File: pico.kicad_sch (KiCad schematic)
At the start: 43 parts, among them J101 Programming, J102 ???, J103 XT60, J104 Conn_01x03, Q101 AGM30P100D, Q102 BSS138, Q103 AGM30P100D, Q104 AGM30P100D, Q105 AGM30P100D, Q106 AGM30P100D, U101 TPS7A2033PDBVR, U106 ADC124S051CIMM/NOPB

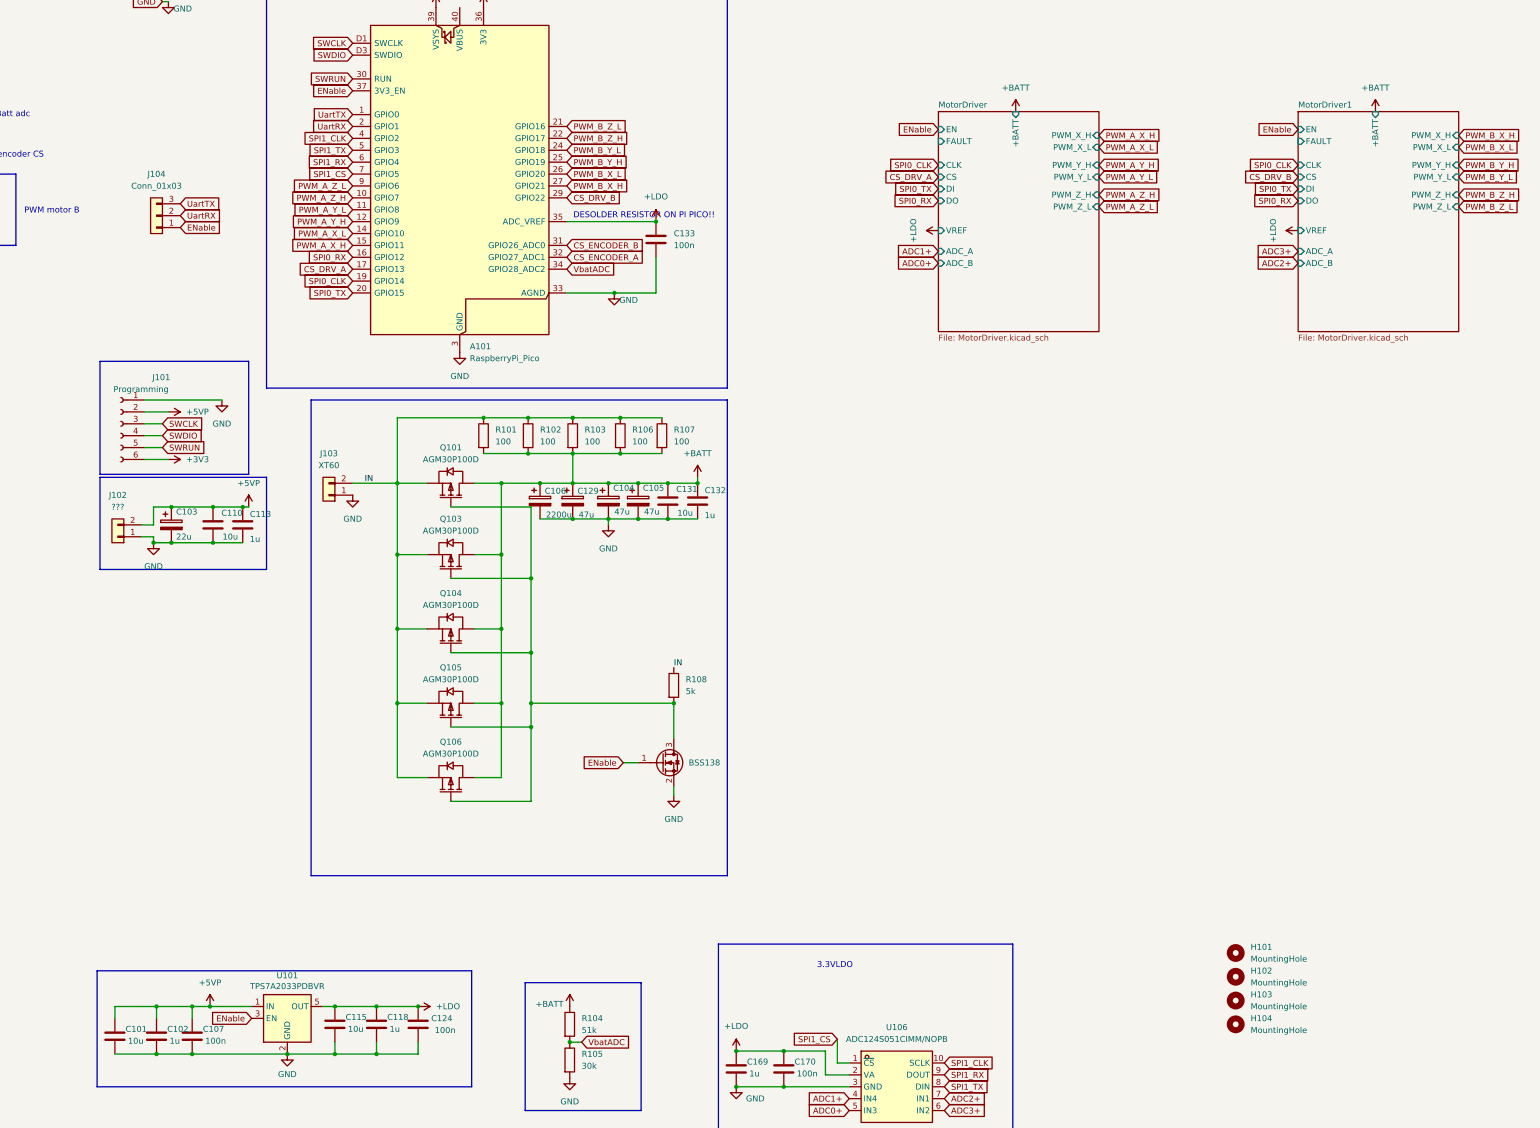
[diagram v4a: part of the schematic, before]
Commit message: done?
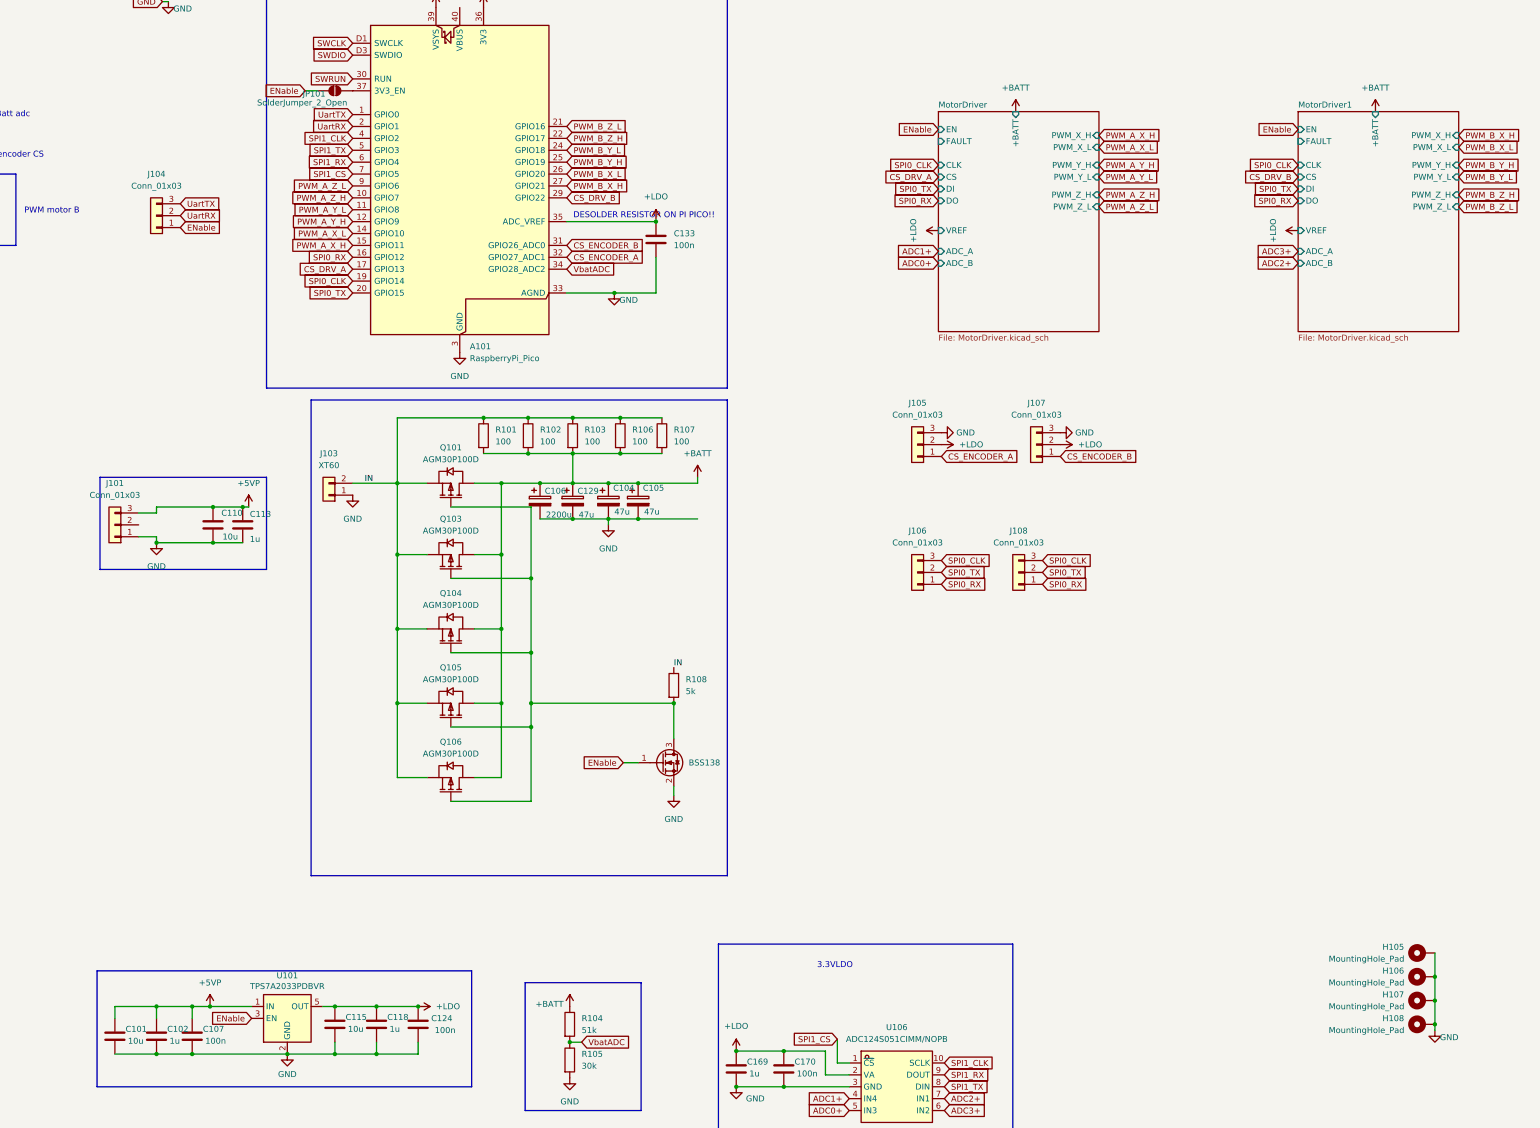
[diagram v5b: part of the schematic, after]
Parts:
- removed C103: 22u, Capacitor_THT:CP_Radial_D5.0mm_P2.00mm, symbol Device:C_Polarized
- removed C131: 10u, COMPONENTS:1206_Resistor, symbol Device:C
- removed C132: 1u, COMPONENTS:1206_Resistor, symbol Device:C
- removed H101, H102, H103, H104: MountingHole, MountingHole:MountingHole_3.2mm_M3, symbol Mechanical:MountingHole
- removed J101: Programming, Connector_PinHeader_2.54mm:PinHeader_1x06_P2.54mm_Vertical, symbol Connector:Conn_01x06_Socket
- removed J102: ???, Connector_PinHeader_2.54mm:PinHeader_1x02_P2.54mm_Vertical, symbol Connector_Generic:Conn_01x02
- added H105, H106, H107, H108: MountingHole_Pad, MountingHole:MountingHole_3.2mm_M3_Pad_Via, symbol Mechanical:MountingHole_Pad
- added J101, J105, J106, J107, J108: Conn_01x03, Connector_JST:JST_XH_B3B-XH-A_1x03_P2.50mm_Vertical, symbol Connector_Generic:Conn_01x03
- added JP101: SolderJumper_2_Open, Jumper:SolderJumper-2_P1.3mm_Open_RoundedPad1.0x1.5mm, symbol Jumper:SolderJumper_2_Open
- J104: footprint Connector_JST:JST_EH_B3B-EH-A_1x03_P2.50mm_Vertical -> Connector_JST:JST_XH_B3B-XH-A_1x03_P2.50mm_Vertical
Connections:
- net +5VP: now also J101.3 (Pin_3)
- net +LDO: now also J105.2 (Pin_2), J107.2 (Pin_2)
- net CS_ENCODER_A: now also J105.1 (Pin_1)
- net CS_ENCODER_B: now also J107.1 (Pin_1)
- net ENable: now also JP101.1 (A); no longer A101.37 (3V3_EN)
- net GND: now also H105.1, H106.1, H107.1, H108.1, J101.1 (Pin_1), J105.3 (Pin_3), J107.3 (Pin_3)
- net SPI0_CLK: now also J106.3 (Pin_3), J108.3 (Pin_3)
- net SPI0_RX: now also J106.1 (Pin_1), J108.1 (Pin_1)
- net SPI0_TX: now also J106.2 (Pin_2), J108.2 (Pin_2)
- new net: A101.37 (3V3_EN), JP101.2 (B)
